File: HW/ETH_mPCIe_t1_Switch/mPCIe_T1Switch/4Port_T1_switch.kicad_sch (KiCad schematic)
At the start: 30 parts, among them U301 LAN9370-V/KCXVAO, U302 TPS62A01

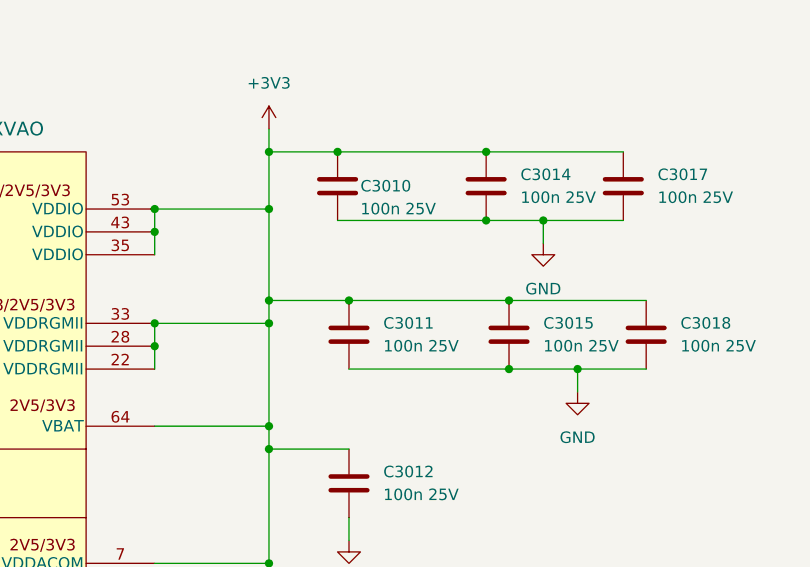
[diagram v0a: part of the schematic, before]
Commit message: .
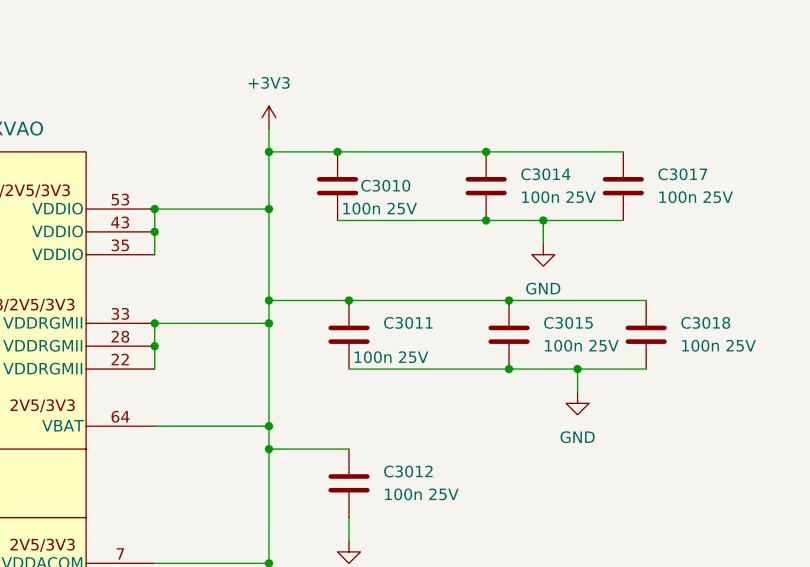
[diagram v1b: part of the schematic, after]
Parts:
- C3001, C3002, C3003, C3004, C3005, C3006, C3007, C3008, C3009, C3010, C3011, C3012, C3013, C3014, C3015, C3016, C3017, C3018, C3019, C3020: footprint Capacitor_SMD:C_0603_1608Metric -> Capacitor_SMD:C_0402_1005Metric; symbol bt_capacitor:C;M;100n;10p;25V;S;0603 -> bt_capacitor:C;M;100n;10p;16V;S;0402; CPN BT00008-091000 -> BT00024-091000; MPN C;M;100n;10p;25V;S;0603 -> C;M;100n;10p;16V;S;0402
